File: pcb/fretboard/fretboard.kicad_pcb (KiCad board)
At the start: 2 copper layers, 46 x 186 mm, 101 parts, among them J1 Conn_01x05_Pin, J10 Conn_01x01_Pin, J11 Conn_01x01_Pin, J12 Conn_01x01_Pin, J13 Conn_01x01_Pin, J14 Conn_01x01_Pin, J15 Conn_01x01_Pin, J16 Conn_01x01_Pin, J17 Conn_01x01_Pin, J18 Conn_01x01_Pin, J19 Conn_01x01_Pin, J2 Conn_01x01_Pin, J20 Conn_01x01_Pin, J21 Conn_01x01_Pin, J22 Conn_01x01_Pin, J23 Conn_01x01_Pin, J24 Conn_01x01_Pin, J25 Conn_01x01_Pin, J26 Conn_01x01_Pin, J27 Conn_01x01_Pin, J28 Conn_01x01_Pin, J29 Conn_01x01_Pin, J3 Conn_01x01_Pin, J30 Conn_01x01_Pin, J31 Conn_01x01_Pin, J32 Conn_01x01_Pin, J33 Conn_01x01_Pin, J34 Conn_01x01_Pin, J35 Conn_01x01_Pin, J36 Conn_01x01_Pin, J37 Conn_01x01_Pin, J38 Conn_01x01_Pin, J39 Conn_01x01_Pin, J4 Conn_01x01_Pin, J40 Conn_01x01_Pin, J41 Conn_01x01_Pin, J42 Conn_01x01_Pin, J43 Conn_01x01_Pin, J44 Conn_01x01_Pin, J45 Conn_01x01_Pin, J46 Conn_01x01_Pin, J47 Conn_01x01_Pin, J48 Conn_01x01_Pin, J49 Conn_01x01_Pin, J5 Conn_01x01_Pin, J50 Conn_01x01_Pin, J51 Conn_01x01_Pin, J52 Conn_01x01_Pin, J53 Conn_01x01_Pin, J54 Conn_01x01_Pin, J55 Conn_01x01_Pin, J56 Conn_01x01_Pin, J57 Conn_01x01_Pin, J58 Conn_01x01_Pin, J59 Conn_01x01_Pin, J6 Conn_01x01_Pin, J60 Conn_01x01_Pin, J61 Conn_01x01_Pin, J7 Conn_01x01_Pin, J8 Conn_01x01_Pin, J9 Conn_01x01_Pin, U1 74HC165, U2 74HC165, U3 74HC165, U4 74HC165

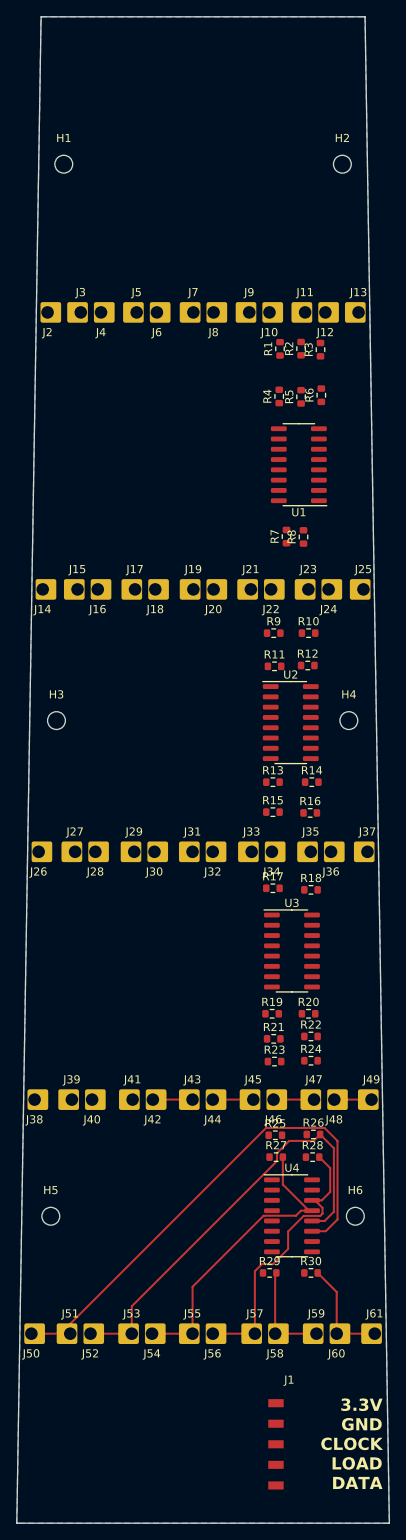
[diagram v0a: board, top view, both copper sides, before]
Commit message: faffing with fretboard
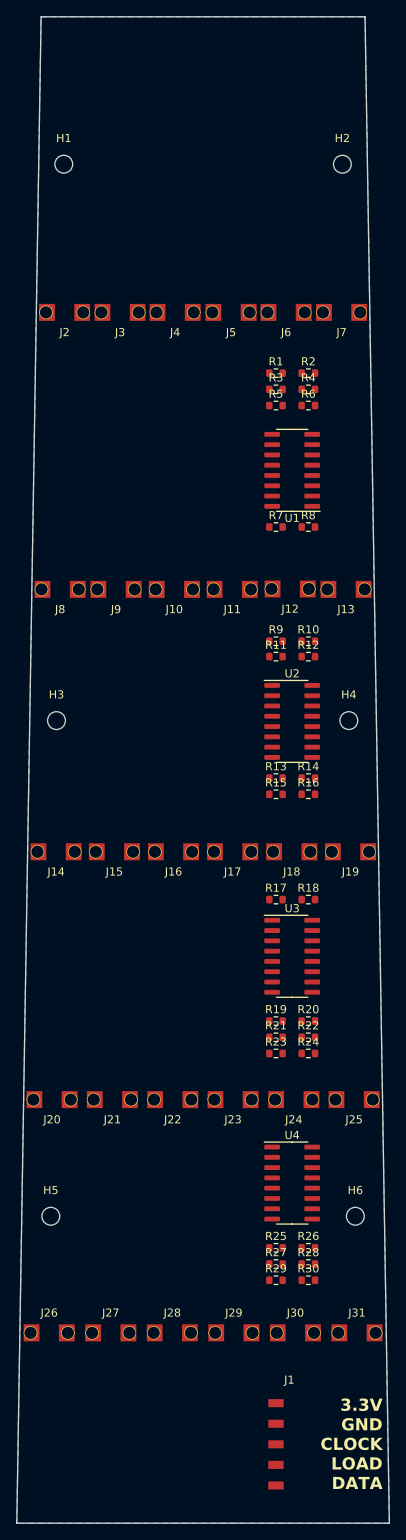
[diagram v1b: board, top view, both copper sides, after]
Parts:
- removed the J11 at (32.6, 36.5)
- removed the J13 at (39.2, 36.5)
- removed the J15 at (4.50, 70.7)
- removed the J17 at (11.6, 70.7)
- removed the J19 at (18.8, 70.7)
- removed the J21 at (25.9, 70.7)
- removed the J23 at (33.0, 70.7)
- removed the J25 at (39.8, 70.7)
- removed the J3 at (4.90, 36.5)
- removed J33, J35, J37, J39, J41, J43, J45, J47, J49, J50, J51, J52, J53, J54, J55, J56, J57, J58, J59, J60, J61: Conn_01x01_Pin, Bjarkar:Bjarkar_fret_connection
- removed the J5 at (11.8, 36.5)
- removed the J7 at (18.8, 36.5)
- removed the J9 at (25.7, 36.5)
- added J26: Conn_01x01_Pin, Bjarkar:Bjarkar_fret_connection, F.Cu at (1.00, 162.5)
- added J28: Conn_01x01_Pin, Bjarkar:Bjarkar_fret_connection, F.Cu at (16.2, 162.5)
- added J30: Conn_01x01_Pin, Bjarkar:Bjarkar_fret_connection, F.Cu at (31.4, 162.5)
- moved J31 62.8 mm to (39.0, 162.5)
- moved J29 60.7 mm to (23.8, 162.5)
- moved J27 59.6 mm to (8.60, 162.5)
- moved R26 14.0 mm to (33.0, 152.0)
- moved R25 13.9 mm to (29.0, 152.0)
- moved R28 13.2 mm to (33.0, 154.0)
- moved R27 13.2 mm to (29.0, 154.0)
- moved R3 7.37 mm to (29.0, 46.0), turned to 0 degrees
- moved U4 4.05 mm to (31.0, 144.0)
- moved R4 3.70 mm to (33.0, 46.0), turned to 0 degrees
- moved R5 3.28 mm to (29.0, 48.0), turned to 0 degrees
- moved R2 3.16 mm to (33.0, 44.0), turned to 0 degrees
- moved R1 3.04 mm to (29.0, 44.0), turned to 0 degrees
- moved J21 2.50 mm to (8.80, 133.7)
- moved J23 2.50 mm to (23.7, 133.7)
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- renumbered J18 to J10, J20 to J11, J22 to J12, J24 to J13, J26 to J14, J28 to J15, J30 to J16, J32 to J17, J34 to J18, J36 to J19, J38 to J20, J40 to J21, J42 to J22, J44 to J23, J46 to J24, J48 to J25, J4 to J3, J6 to J4, J8 to J5, J10 to J6, J12 to J7, J14 to J8, J16 to J9
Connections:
- J14 pad 1: Net-(J26-Pin_1) (its old number) -> Net-(J14-Pin_1)
- J15 pad 1: Net-(J28-Pin_1) (its old number) -> Net-(J15-Pin_1)
- J16 pad 1: Net-(J30-Pin_1) (its old number) -> Net-(J16-Pin_1)
- J27 pad 1: Net-(J26-Pin_1) (its old number) -> Net-(J27-Pin_1)
- J29 pad 1: Net-(J28-Pin_1) (its old number) -> Net-(J29-Pin_1)
- J31 pad 1: Net-(J30-Pin_1) (its old number) -> Net-(J31-Pin_1)
- R13 pad 2: Net-(J26-Pin_1) (its old number) -> Net-(J14-Pin_1)
- R14 pad 2: Net-(J28-Pin_1) (its old number) -> Net-(J15-Pin_1)
- R15 pad 2: Net-(J30-Pin_1) (its old number) -> Net-(J16-Pin_1)
- R26 pad 2: Net-(J52-Pin_1) -> Net-(J27-Pin_1)
- R28 pad 2: Net-(J56-Pin_1) -> Net-(J29-Pin_1)
- R30 pad 2: Net-(J60-Pin_1) -> Net-(J31-Pin_1)
- U2 pad 3: Net-(J26-Pin_1) (its old number) -> Net-(J14-Pin_1)
- U2 pad 4: Net-(J28-Pin_1) (its old number) -> Net-(J15-Pin_1)
- U2 pad 5: Net-(J30-Pin_1) (its old number) -> Net-(J16-Pin_1)
- U4 pad 12: Net-(J52-Pin_1) -> Net-(J27-Pin_1)
- U4 pad 14: Net-(J56-Pin_1) -> Net-(J29-Pin_1)
- U4 pad 4: Net-(J60-Pin_1) -> Net-(J31-Pin_1)
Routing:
- net Net-(J26-Pin_1): track 63.1 -> 0.00 mm
- net Net-(J52-Pin_1): track 54.5 -> 0.00 mm
- net Net-(J28-Pin_1): track 37.8 -> 0.00 mm
- net Net-(J56-Pin_1): track 35.4 -> 0.00 mm
- net Net-(J60-Pin_1): track 13.2 -> 0.00 mm
- net Net-(J30-Pin_1): track 12.7 -> 0.00 mm
- net Net-(J24-Pin_1): track 5.00 -> 0.00 mm
- net Net-(J23-Pin_1): track 5.00 -> 0.00 mm
- net Net-(J22-Pin_1): track 4.90 -> 0.00 mm
- net Net-(J25-Pin_1): track 4.60 -> 0.00 mm
